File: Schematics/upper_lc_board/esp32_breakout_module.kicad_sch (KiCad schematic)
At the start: 28 parts, among them J1 USB_C_Female_USB2_Small, Q4 2N7002, SW1 SW_ESP_BOOT_MODE, SW2 SW_ESP_RESET, U1 ESP32-S3-WROOM-1-N16, U2 ISO1044BDR

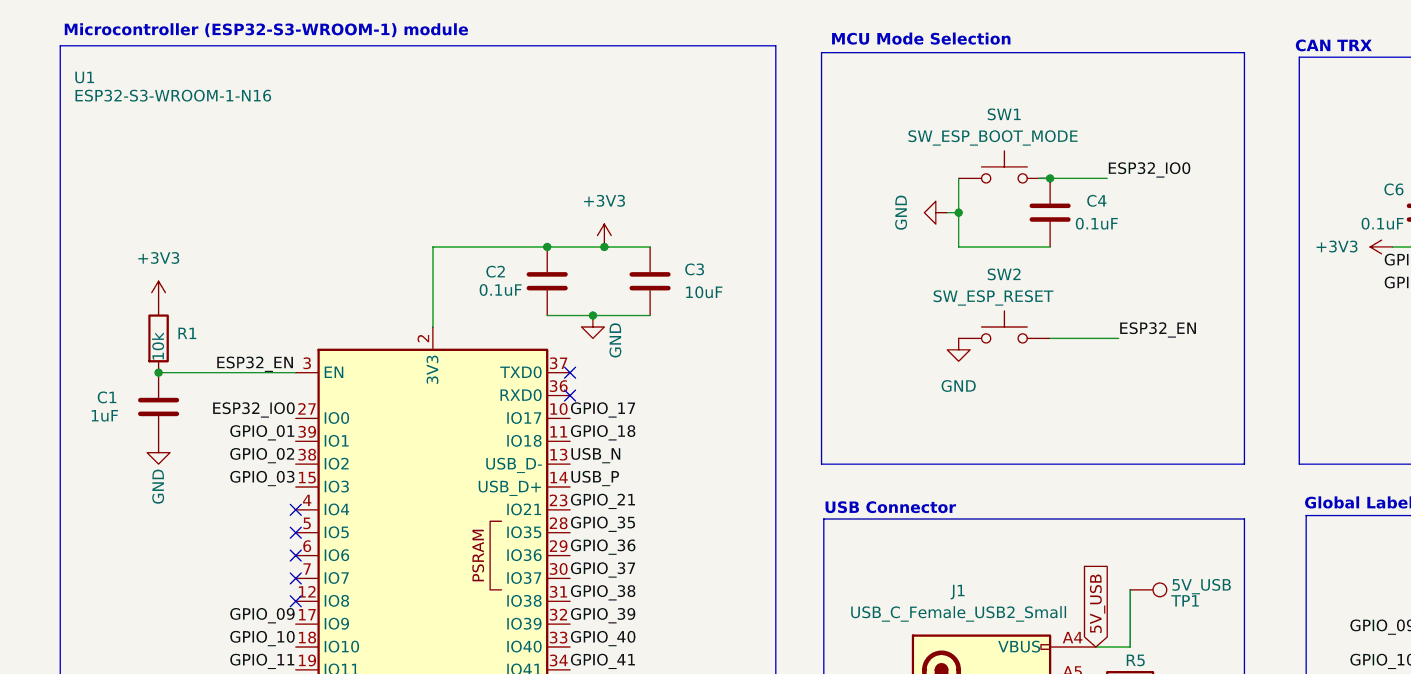
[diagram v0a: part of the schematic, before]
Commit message: final upper control board
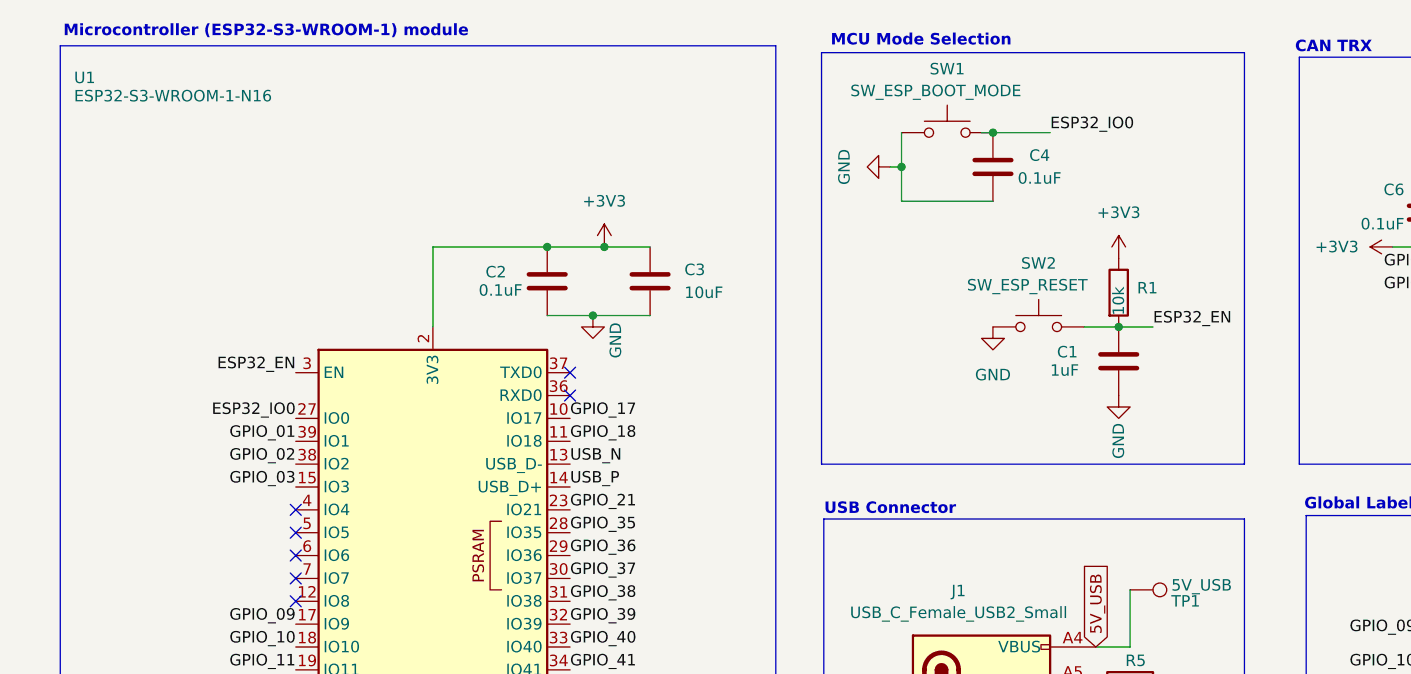
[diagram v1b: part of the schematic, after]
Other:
- moved on the sheet: C4, SW1, SW2
